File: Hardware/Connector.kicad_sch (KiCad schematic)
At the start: 14 parts, among them J1 XIAO ESP32S3 Sense, J2 Conn_02x16_Counter_Clockwise, J3 FTSH-107-01-L-D-K

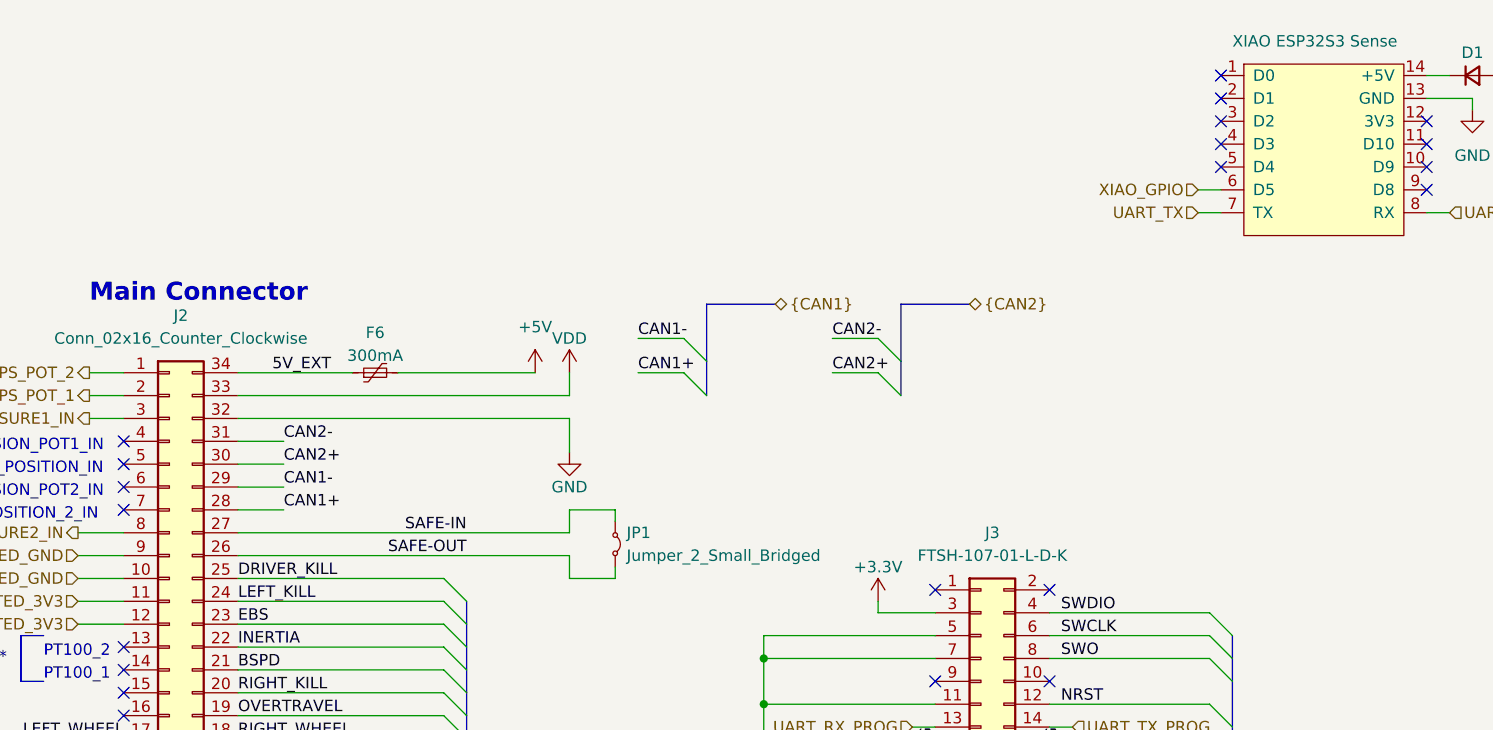
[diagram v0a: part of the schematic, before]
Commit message: BOM update
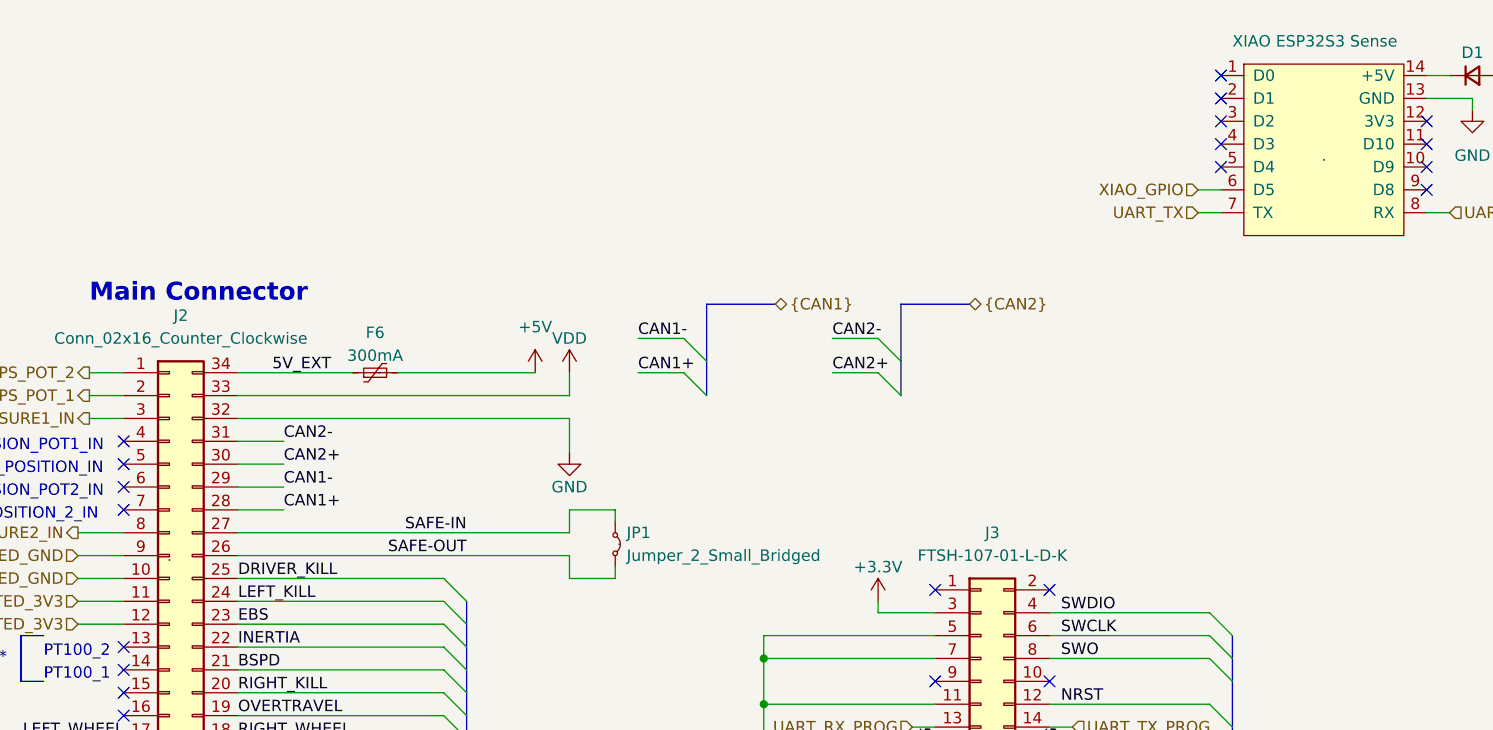
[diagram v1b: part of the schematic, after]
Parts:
- D3: Mouser Part Number (none) -> 637-BZX84C5V6
- D4: Mouser Part Number (none) -> 78-BZX84C3V6-E3-08
- D7, D8: Mouser Part Number (none) -> 771-PESD5V0L2BT-QR
- F6, J1, J2, JP1: Mouser Part Number (none) -> .
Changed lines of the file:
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@@
+			)
+		)
+		(property "Mouser Part Number" "771-PESD5V0L2BT-QR"
+			(at 139.7 153.67 0)
+			(effects
+				(font
+					(size 1.27 1.27)
+				)
+				(hide yes)
 			)
 		)
@@
 			)
 		)
+		(property "Mouser Part Number" "771-PESD5V0L2BT-QR"
+			(at 171.45 153.67 0)
+			(effects
+				(font
+					(size 1.27 1.27)
+				)
+				(hide yes)
+			)
+		)
 		(pin "1"
 		)
@@
 			)
 		)
+		(property "Mouser Part Number" "78-BZX84C3V6-E3-08"
+			(at 245.11 143.51 0)
+			(effects
+				(font
+					(size 1.27 1.27)
+				)
+				(hide yes)
+			)
+		)
 		(pin "1"
 		)
@@
 			)
 		)
+		(property "Mouser Part Number" "."
+			(at 144.78 72.39 0)
+			(effects
+				(font
+					(size 1.27 1.27)
+				)
+			)
+		)
 		(pin "1"
 		)
@@
 			)
 		)
+		(property "Mouser Part Number" "."
+			(at 171.45 91.44 0)
+			(effects
+				(font
+					(size 1.27 1.27)
+				)
+			)
+		)
 		(pin "1"
 		)
@@
 			)
 		)
+		(property "Mouser Part Number" "."
+			(at 121.92 92.71 0)
+			(effects
+				(font
+					(size 1.27 1.27)
+				)
+			)
+		)
 		(pin "1"
 		)
@@
 			)
 		)
+		(property "Mouser Part Number" "637-BZX84C5V6"
+			(at 190.5 143.51 0)
+			(effects
+				(font
+					(size 1.27 1.27)
+				)
+				(hide yes)
+			)
+		)
 		(pin "1"
 		)
@@
 			)
 		)
+		(property "Mouser Part Number" "."
+			(at 250.19 48.26 0)
+			(effects
+				(font
+					(size 1.27 1.27)
+				)
+			)
+		)
